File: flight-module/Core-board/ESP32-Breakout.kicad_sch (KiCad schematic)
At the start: 21 parts, among them P1 USB_C_Plug_USB2.0, SW2 SW_MEC_5E, SW3 SW_MEC_5E, U1 ESP32-S3-WROOM-1-N16R2, U4 AZ1084-3.3

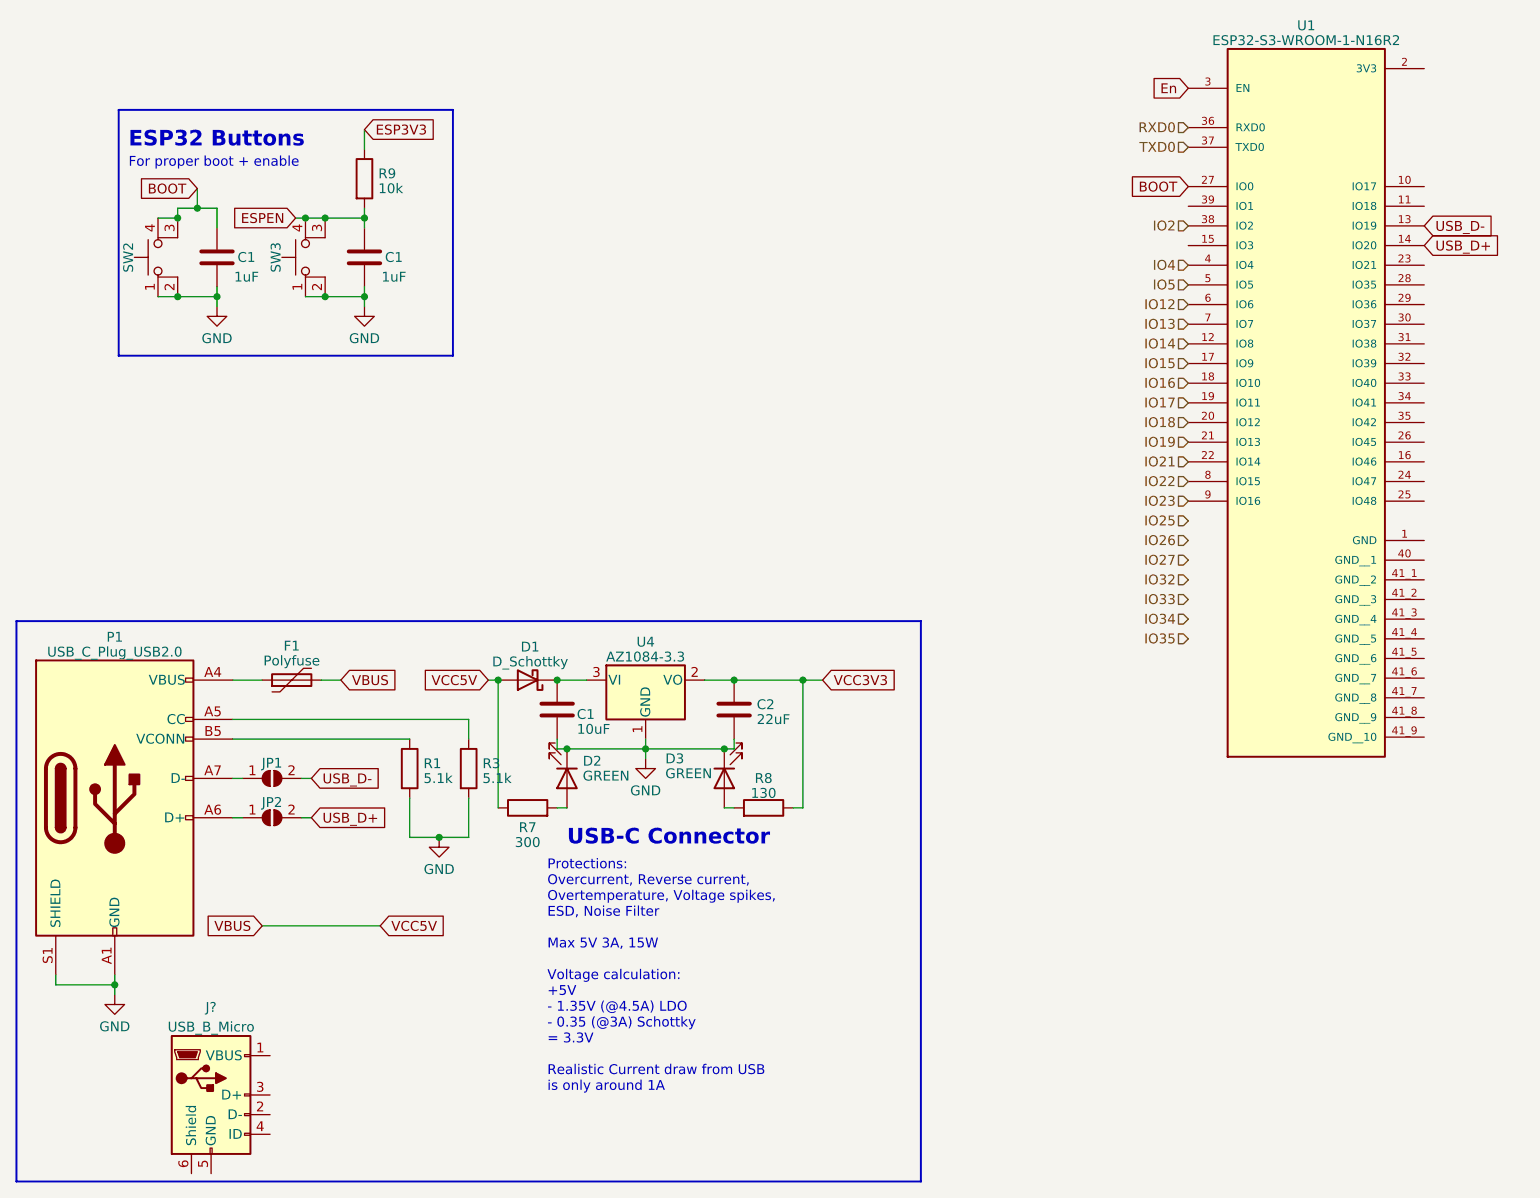
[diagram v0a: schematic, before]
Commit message: Updated core-board
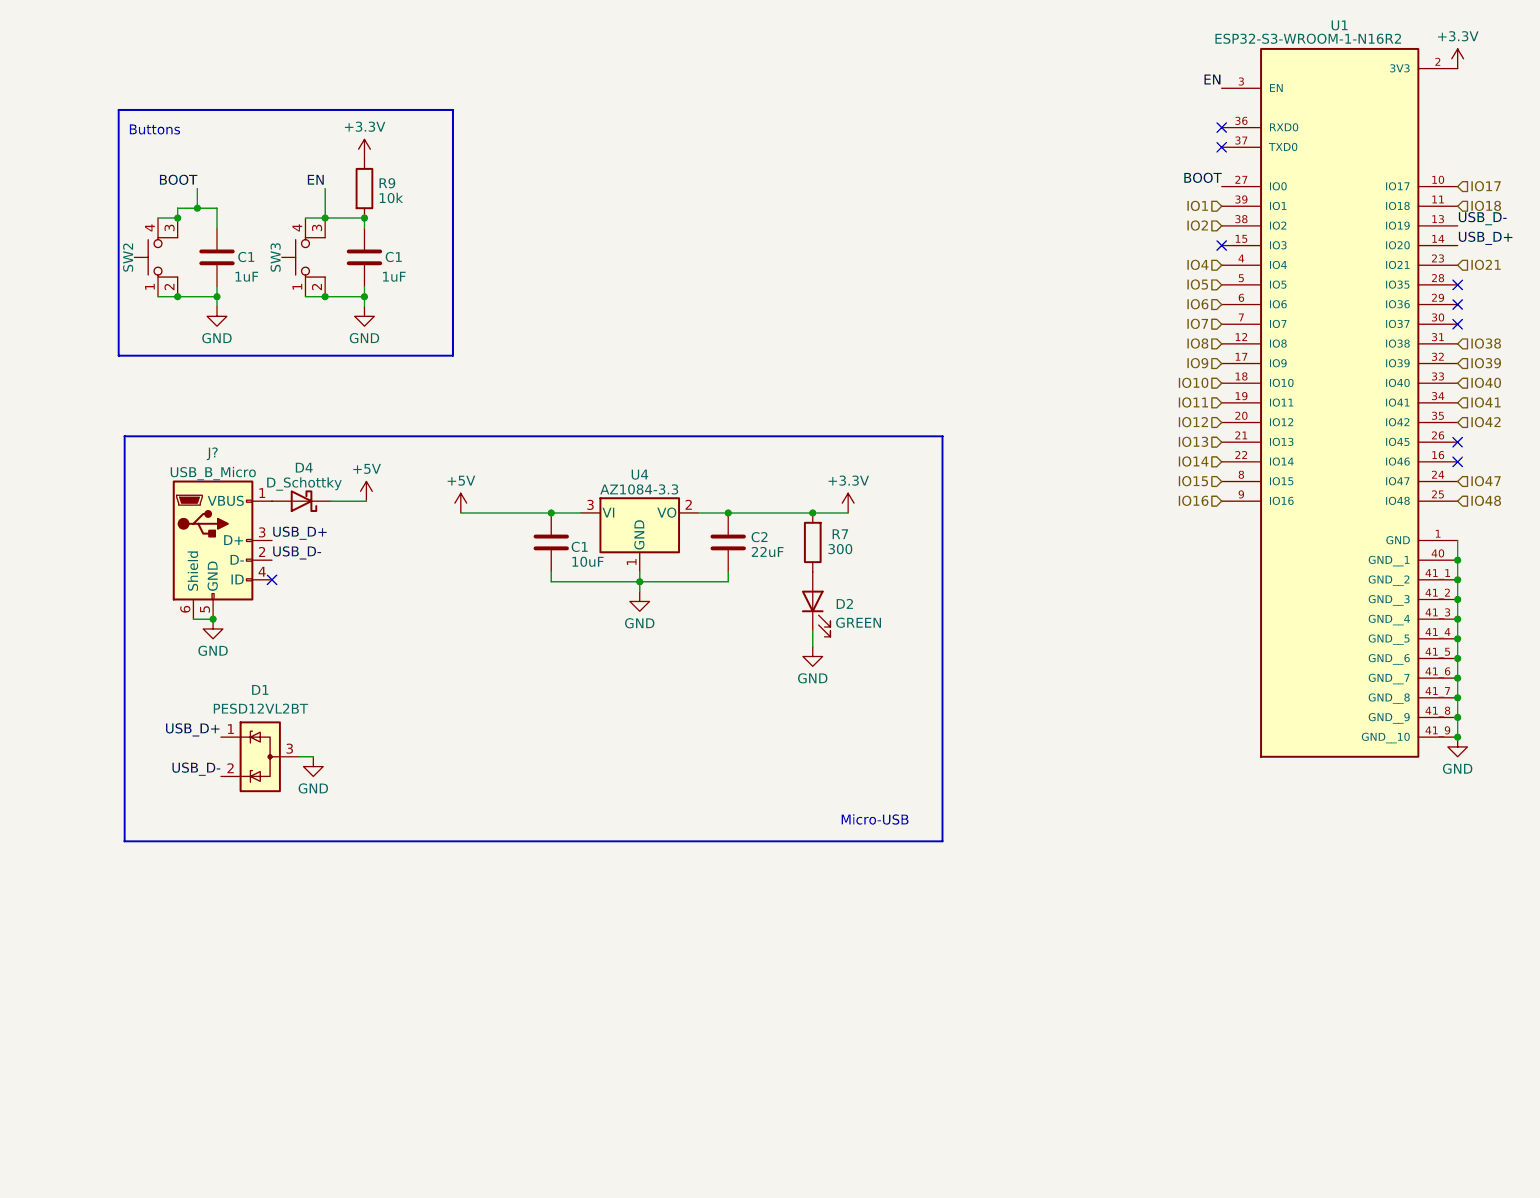
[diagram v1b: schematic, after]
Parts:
- removed D1: D_Schottky, Diode_SMD:D_SOD-128, symbol Device:D_Schottky
- removed D3: GREEN, LED_SMD:LED_1206_3216Metric_Pad1.42x1.75mm_HandSolder, symbol Device:LED
- removed F1: Polyfuse, Fuse:Fuse_1812_4532Metric_Pad1.30x3.40mm_HandSolder, symbol Device:Polyfuse
- removed JP1, JP2: ~, Jumper:SolderJumper-2_P1.3mm_Open_RoundedPad1.0x1.5mm, symbol Jumper:SolderJumper_2_Open
- removed P1: USB_C_Plug_USB2.0, Connector_USB:USB_C_Receptacle_GCT_USB4085, symbol Connector:USB_C_Plug_USB2.0
- removed R1, R3: 5.1k, Resistor_SMD:R_0805_2012Metric_Pad1.20x1.40mm_HandSolder, symbol Device:R
- removed R8: 130, Resistor_SMD:R_0805_2012Metric_Pad1.20x1.40mm_HandSolder, symbol Device:R
- added D1: PESD12VL2BT, Package_TO_SOT_SMD:SOT-23, symbol Power_Protection:SP0502BAHT
- added D4: D_Schottky, Diode_SMD:D_SOD-128, symbol Device:D_Schottky
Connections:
- net ESP3V3 is gone; now on net +3.3V: R9.1
- net En is gone; now on net EN: U1.3 (EN)
- net IO19 is gone; now on net IO13: U1.21 (IO13)
- net IO22 is gone; now on net IO15: U1.8 (IO15)
- net IO23 is gone; now on net IO16: U1.9 (IO16)
- net VBUS is gone; now on an unnamed net: R7.1
- net VCC3V3 is gone; now on net +3.3V: C2.1, U4.2 (VO)
- net GND: now also J?.5 (GND), J?.6 (Shield), U1.1 (GND), U1.40 (GND__1), U1.41_1 (GND__2), U1.41_2 (GND__3), U1.41_3 (GND__4), U1.41_4 (GND__5), U1.41_5 (GND__6), U1.41_6 (GND__7), U1.41_7 (GND__8), U1.41_8 (GND__9), U1.41_9 (GND__10), D1.3 (A)
- net IO12: now also U1.20 (IO12); no longer U1.6 (IO6)
- net IO13: no longer U1.7 (IO7)
- net IO14: now also U1.22 (IO14); no longer U1.12 (IO8)
- net IO15: no longer U1.17 (IO9)
- net IO16: no longer U1.18 (IO10)
- net IO17: now also U1.10 (IO17); no longer U1.19 (IO11)
- net IO18: now also U1.11 (IO18); no longer U1.20 (IO12)
- net IO21: now also U1.23 (IO21); no longer U1.22 (IO14)
- net USB_D+: now also J?.3 (D+), D1.1 (K)
- net USB_D-: now also J?.2 (D-), D1.2 (K)
- net +3.3V: now reaches U1.2 (3V3)
- net +3.3V: now also R7.2
- net IO47: now reaches U1.24 (IO47)
- net IO48: now reaches U1.25 (IO48)
- net IO38: now reaches U1.31 (IO38)
- net IO39: now reaches U1.32 (IO39)
- net IO40: now reaches U1.33 (IO40)
- net IO41: now reaches U1.34 (IO41)
- net IO42: now reaches U1.35 (IO42)
- net IO1: now reaches U1.39 (IO1)
- net +5V: now reaches C1.1, U4.3 (VI)
- net +5V: now also D4.1 (K)
- net at D2.2 (A): no longer R7.2
- net at J?.1 (VBUS): now also D4.2 (A)
- net ESPEN renamed EN
- net RXD0: no longer names the net of U1.36 (RXD0)
- net TXD0: no longer names the net of U1.37 (TXD0)
- new net IO10: U1.18 (IO10)
- new net IO11: U1.19 (IO11)
- new net IO6: U1.6 (IO6)
- new net IO7: U1.7 (IO7)
- new net IO8: U1.12 (IO8)
- new net IO9: U1.17 (IO9)
- no-connect marks 0 -> 9
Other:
- note added: "Buttons"
- note added: "Micro-USB"
- note removed: "ESP32 Buttons"
- note removed: "For proper boot + enable"
- note removed: "Protections: Overcurrent, Reverse current, Overtemperature, Voltage spikes, ESD, Noise Filter Max 5V 3A, 15W Voltage calculation: +5V - 1.35V (@4.5A) LDO - 0.35 (@3A) Schottky = 3.3V Realistic Current draw from USB is only around 1A"
- note removed: "USB-C Connector"
- moved on the sheet: C1, C2, D2, J?, R7, R9, U1, U4
